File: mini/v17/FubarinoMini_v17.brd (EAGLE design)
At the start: 50.8 x 17.8 mm, 36 parts, among them IC1 AP7215-33YG-13, J1 M20, J2 M20, J8 USB-5PIN, Q1 8MHz, Q2 32.768 KHz, U1 PIC32MX270F256D_44QFN_44

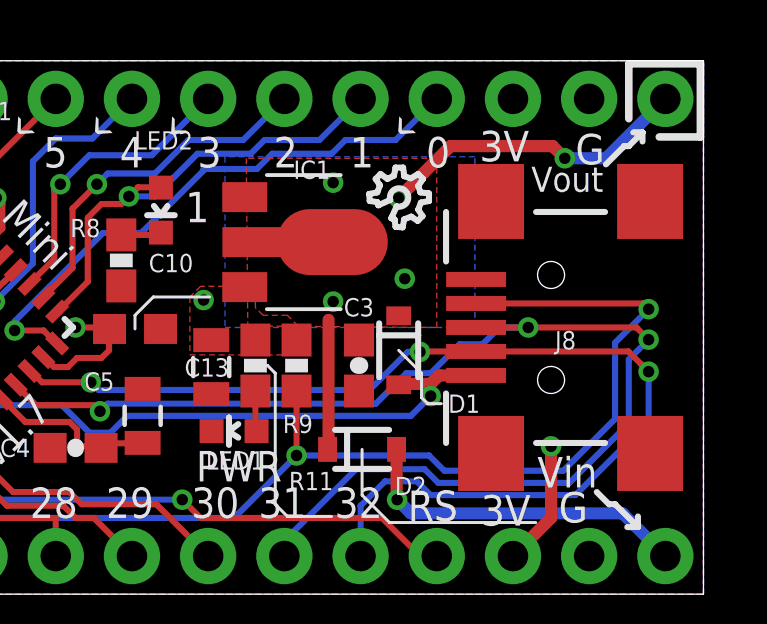
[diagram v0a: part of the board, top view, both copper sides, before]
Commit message: v1.7 updates.
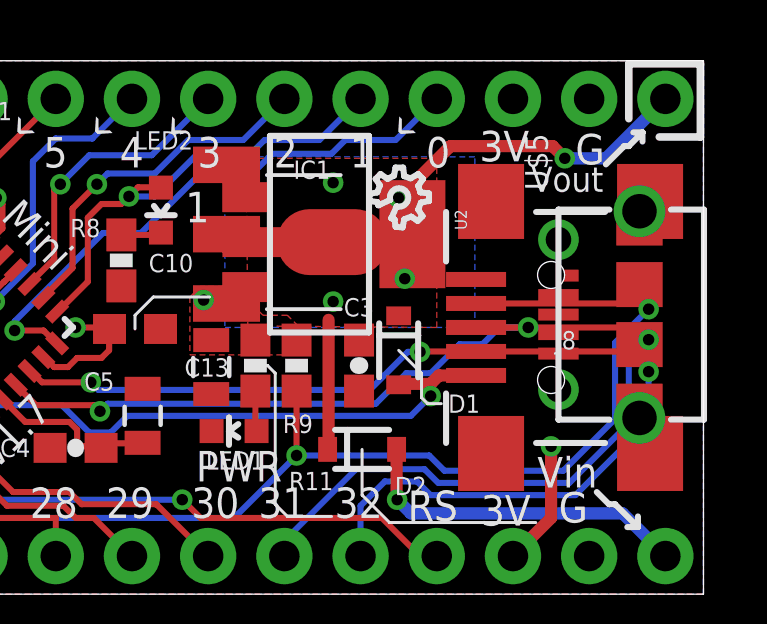
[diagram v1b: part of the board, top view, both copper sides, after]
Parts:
- added U$5: USBMICROB, SchmalzHaus:USB-MICROB_FCI_PINS
- added U2: (no value), SparkFun-IC-Power:SOT223
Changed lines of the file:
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@@
 <?xml version="1.0" encoding="utf-8"?>
 <!DOCTYPE eagle SYSTEM "eagle.dtd">
-<eagle version="9.0.0">
+<eagle version="9.0.1">
 <drawing>
 <settings>
@@
 <layer number="15" name="Route15" color="4" fill="6" visible="no" active="no"/>
 <layer number="16" name="Bottom" color="1" fill="1" visible="no" active="yes"/>
-<layer number="17" name="Pads" color="2" fill="1" visible="no" active="yes"/>
-<layer number="18" name="Vias" color="2" fill="1" visible="no" active="yes"/>
+<layer number="17" name="Pads" color="2" fill="1" visible="yes" active="yes"/>
+<layer number="18" name="Vias" color="2" fill="1" visible="yes" active="yes"/>
 <layer number="19" name="Unrouted" color="14" fill="1" visible="no" active="yes"/>
-<layer number="20" name="Dimension" color="15" fill="1" visible="no" active="yes"/>
-<layer number="21" name="tPlace" color="16" fill="1" visible="no" active="yes"/>
+<layer number="20" name="Dimension" color="15" fill="1" visible="yes" active="yes"/>
+<layer number="21" name="tPlace" color="16" fill="1" visible="yes" active="yes"/>
 <layer number="22" name="bPlace" color="15" fill="1" visible="no" active="yes"/>
 <layer number="23" name="tOrigins" color="15" fill="1" visible="yes" active="yes"/>
@@
 <layer number="54" name="bGND_GNDA" color="1" fill="9" visible="no" active="yes"/>
 <layer number="56" name="wert" color="7" fill="1" visible="no" active="no"/>
+<layer number="57" name="tCAD" color="7" fill="1" visible="no" active="no"/>
+<layer number="59" name="tCarbon" color="7" fill="1" visible="no" active="no"/>
+<layer number="60" name="bCarbon" color="7" fill="1" visible="no" active="no"/>
+<layer number="90" name="Modules" color="5" fill="1" visible="no" active="no"/>
 <layer number="91" name="Nets" color="2" fill="1" visible="no" active="no"/>
 <layer number="92" name="Busses" color="1" fill="1" visible="no" active="no"/>
@@
 <layer number="97" name="Info" color="7" fill="1" visible="no" active="no"/>
 <layer number="98" name="Guide" color="6" fill="1" visible="no" active="no"/>
+<layer number="99" name="SpiceOrder" color="7" fill="1" visible="no" active="no"/>
 <layer number="100" name="Muster" color="7" fill="1" visible="no" active="no"/>
 <layer number="101" name="Patch_Top" color="12" fill="4" visible="no" active="no"/>
@@
 <layer number="106" name="bPlate" color="7" fill="1" visible="no" active="yes"/>
 <layer number="107" name="Crop" color="7" fill="1" visible="no" active="yes"/>
+<layer number="108" name="tplace-old" color="10" fill="1" visible="yes" active="yes"/>
+<layer number="109" name="ref-old" color="11" fill="1" visible="yes" active="yes"/>
+<layer number="110" name="fp0" color="7" fill="1" visible="yes" active="yes"/>
+<layer number="111" name="LPC17xx" color="7" fill="1" visible="yes" active="yes"/>
+<layer number="112" name="tSilk" color="7" fill="1" visible="yes" active="yes"/>
+<layer number="113" name="IDFDebug" color="4" fill="1" visible="yes" active="yes"/>
+<layer number="114" name="Badge_Outline" color="7" fill="1" visible="yes" active="yes"/>
+<layer number="115" name="ReferenceISLANDS" color="7" fill="1" visible="yes" active="yes"/>
 <layer number="116" name="Patch_BOT" color="9" fill="4" visible="no" active="no"/>
+<layer number="118" name="Rect_Pads" color="7" fill="1" visible="yes" active="yes"/>
 <layer number="121" name="_tsilk" color="14" fill="1" visible="no" active="yes"/>
 <layer number="122" name="_bsilk" color="14" fill="1" visible="no" active="yes"/>
+<layer number="123" name="tTestmark" color="7" fill="1" visible="yes" active="yes"/>
+<layer number="124" name="bTestmark" color="7" fill="1" visible="yes" active="yes"/>
 <layer number="125" name="_tNames" color="7" fill="1" visible="no" active="yes"/>
+<layer number="126" name="_bNames" color="7" fill="1" visible="yes" active="yes"/>
+<layer number="127" name="_tValues" color="7" fill="1" visible="yes" active="yes"/>
 <layer number="128" name="128bmp" color="7" fill="1" visible="no" active="yes"/>
 <layer number="129" name="129bmp" color="7" fill="1" visible="no" active="yes"/>
 <layer number="130" name="130bmp" color="7" fill="1" visible="no" active="yes"/>
+<layer number="131" name="tAdjust" color="7" fill="1" visible="yes" active="yes"/>
+<layer number="132" name="bAdjust" color="7" fill="1" visible="yes" active="yes"/>
 <layer number="144" name="DrillLegend" color="7" fill="1" visible="no" active="yes"/>
 <layer number="145" name="DrillLegend_01-16" color="2" fill="9" visible="no" active="yes"/>
 <layer number="146" name="DrillLegend_01-20" color="3" fill="9" visible="no" active="yes"/>
+<layer number="150" name="Notes" color="7" fill="1" visible="yes" active="yes"/>
 <layer number="151" name="HeatSink" color="7" fill="1" visible="no" active="no"/>
+<layer number="152" name="_bDocu" color="7" fill="1" visible="yes" active="yes"/>
+<layer number="153" name="FabDoc1" color="7" fill="1" visible="yes" active="yes"/>
+<layer number="154" name="FabDoc2" color="7" fill="1" visible="yes" active="yes"/>
+<layer number="155" name="FabDoc3" color="7" fill="1" visible="yes" active="yes"/>
 <layer number="199" name="Contour" color="7" fill="1" visible="no" active="yes"/>
 <layer number="200" name="200bmp" color="1" fill="10" visible="no" active="no"/>
@@
 <layer number="223" name="223bmp" color="24" fill="1" visible="no" active="no"/>
 <layer number="224" name="224bmp" color="25" fill="1" visible="no" active="no"/>
+<layer number="225" name="225bmp" color="7" fill="1" visible="yes" active="yes"/>
+<layer number="226" name="226bmp" color="7" fill="1" visible="yes" active="yes"/>
+<layer number="227" name="227bmp" color="11" fill="1" visible="yes" active="yes"/>
+<layer number="228" name="228bmp" color="10" fill="1" visible="yes" active="yes"/>
+<layer number="229" name="229bmp" color="14" fill="1" visible="yes" active="yes"/>
+<layer number="230" name="230bmp" color="12" fill="1" visible="yes" active="yes"/>
+<layer number="231" name="231bmp" color="9" fill="1" visible="yes" active="yes"/>
+<layer number="232" name="Eagle3D_PG2" color="7" fill="1" visible="yes" active="yes"/>
+<layer number="233" name="Eagle3D_PG3" color="7" fill="1" visible="yes" active="yes"/>
+<layer number="248" name="Housing" color="7" fill="1" visible="yes" active="yes"/>
+<layer number="249" name="Edge" color="7" fill="1" visible="yes" active="yes"/>
 <layer number="250" name="Descript" color="3" fill="1" visible="no" active="no"/>
 <layer number="251" name="SMDround" color="12" fill="11" visible="no" active="no"/>
 <layer number="254" name="cooling" color="7" fill="1" visible="no" active="no"/>
+<layer number="255" name="routoute" color="7" fill="1" visible="yes" active="yes"/>
 </layers>
 <board>
@@
 </element>
 <element name="DRILEGEND" library="drilegend" package="DRILEGEND" value="" x="101.19484375" y="28.702"/>
+<element name="U2" library="SparkFun-IC-Power" package="SOT223" value="" x="38" y="12" rot="R270">
+<attribute name="PROD_ID" value="VREG-08170" x="38" y="12" size="1.778" layer="27" rot="R270" display="off"/>
+</element>
+<element name="U$5" library="SchmalzHaus" package="USB-MICROB_FCI_PINS" value="USBMICROB" x="48.667" y="9.319" rot="R90"/>
 </elements>
 <signals>
